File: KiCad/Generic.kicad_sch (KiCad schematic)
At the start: 39 parts, among them J1 Connector, J2 USB-C, J3 DC, U1 ESP32-WROOM-32, U2 FT231XQ, U3 LMR16006+FB

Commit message: Library tidy
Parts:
- D3, D4: footprint RevK:SOT-363_SC-70-6 -> Package_TO_SOT_SMD:SOT-363_SC-70-6
- U1: footprint RF_Module:ESP32-WROOM-32 -> RevK:ESP32-WROOM-32
- U2: footprint RevK:QFN-20-1EP_4x4mm_P0.5mm_EP2.5x2.5mm -> Package_DFN_QFN:QFN-20-1EP_4x4mm_P0.5mm_EP2.5x2.5mm
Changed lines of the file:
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@@
     (property "Reference" "U2" (id 0) (at 158.115 139.7 0))
     (property "Value" "FT231XQ" (id 1) (at 170.18 119.38 0))
-    (property "Footprint" "RevK:QFN-20-1EP_4x4mm_P0.5mm_EP2.5x2.5mm" (id 2) (at 205.105 138.43 0)
+    (property "Footprint" "Package_DFN_QFN:QFN-20-1EP_4x4mm_P0.5mm_EP2.5x2.5mm" (id 2) (at 205.105 138.43 0)
       (effects (font (size 1.27 1.27)) hide)
     )
@@
     (property "Reference" "D3" (id 0) (at 239.395 96.0882 0))
     (property "Value" "BAV99S" (id 1) (at 239.395 98.3996 0))
-    (property "Footprint" "RevK:SOT-363_SC-70-6" (id 2) (at 239.395 114.3 0)
+    (property "Footprint" "Package_TO_SOT_SMD:SOT-363_SC-70-6" (id 2) (at 239.395 114.3 0)
       (effects (font (size 1.27 1.27)) hide)
     )
@@
     (property "Reference" "D3" (id 0) (at 239.395 111.3282 0))
     (property "Value" "BAV99S" (id 1) (at 239.395 113.6396 0))
-    (property "Footprint" "RevK:SOT-363_SC-70-6" (id 2) (at 239.395 129.54 0)
+    (property "Footprint" "Package_TO_SOT_SMD:SOT-363_SC-70-6" (id 2) (at 239.395 129.54 0)
       (effects (font (size 1.27 1.27)) hide)
     )
@@
     (property "Reference" "D4" (id 0) (at 239.395 127.2032 0))
     (property "Value" "BAV99S" (id 1) (at 239.395 129.5146 0))
-    (property "Footprint" "RevK:SOT-363_SC-70-6" (id 2) (at 239.395 145.415 0)
+    (property "Footprint" "Package_TO_SOT_SMD:SOT-363_SC-70-6" (id 2) (at 239.395 145.415 0)
       (effects (font (size 1.27 1.27)) hide)
     )
@@
     (property "Reference" "D4" (id 0) (at 239.395 143.7132 0))
     (property "Value" "BAV99S" (id 1) (at 239.395 146.0246 0))
-    (property "Footprint" "RevK:SOT-363_SC-70-6" (id 2) (at 239.395 161.925 0)
+    (property "Footprint" "Package_TO_SOT_SMD:SOT-363_SC-70-6" (id 2) (at 239.395 161.925 0)
       (effects (font (size 1.27 1.27)) hide)
     )
@@
       (effects (font (size 1.27 1.27)) (justify left))
     )
-    (property "Footprint" "RF_Module:ESP32-WROOM-32" (id 2) (at 65.405 105.41 0)
+    (property "Footprint" "RevK:ESP32-WROOM-32" (id 2) (at 65.405 105.41 0)
       (effects (font (size 1.27 1.27)) hide)
     )
@@
     )
     (path "/00000000-0000-0000-0000-0000609f92b0"
-      (reference "D3") (unit 1) (value "BAV99S") (footprint "RevK:SOT-363_SC-70-6")
+      (reference "D3") (unit 1) (value "BAV99S") (footprint "Package_TO_SOT_SMD:SOT-363_SC-70-6")
     )
     (path "/00000000-0000-0000-0000-000060ddc5e7"
-      (reference "D3") (unit 2) (value "BAV99S") (footprint "RevK:SOT-363_SC-70-6")
+      (reference "D3") (unit 2) (value "BAV99S") (footprint "Package_TO_SOT_SMD:SOT-363_SC-70-6")
     )
     (path "/00000000-0000-0000-0000-000060ddef2c"
-      (reference "D4") (unit 1) (value "BAV99S") (footprint "RevK:SOT-363_SC-70-6")
+      (reference "D4") (unit 1) (value "BAV99S") (footprint "Package_TO_SOT_SMD:SOT-363_SC-70-6")
     )
     (path "/00000000-0000-0000-0000-000060de1009"
-      (reference "D4") (unit 2) (value "BAV99S") (footprint "RevK:SOT-363_SC-70-6")
+      (reference "D4") (unit 2) (value "BAV99S") (footprint "Package_TO_SOT_SMD:SOT-363_SC-70-6")
     )
     (path "/00000000-0000-0000-0000-0000610fe5d2"
@@
     )
     (path "/d3737146-f8f2-4cf9-a53d-a4805b531c09"
-      (reference "U1") (unit 1) (value "ESP32-WROOM-32") (footprint "RF_Module:ESP32-WROOM-32")
+      (reference "U1") (unit 1) (value "ESP32-WROOM-32") (footprint "RevK:ESP32-WROOM-32")
     )
     (path "/00000000-0000-0000-0000-000060849d1e"
-      (reference "U2") (unit 1) (value "FT231XQ") (footprint "RevK:QFN-20-1EP_4x4mm_P0.5mm_EP2.5x2.5mm")
+      (reference "U2") (unit 1) (value "FT231XQ") (footprint "Package_DFN_QFN:QFN-20-1EP_4x4mm_P0.5mm_EP2.5x2.5mm")
     )
     (path "/c88f1737-32b5-4cea-a76f-93ad322556d3"

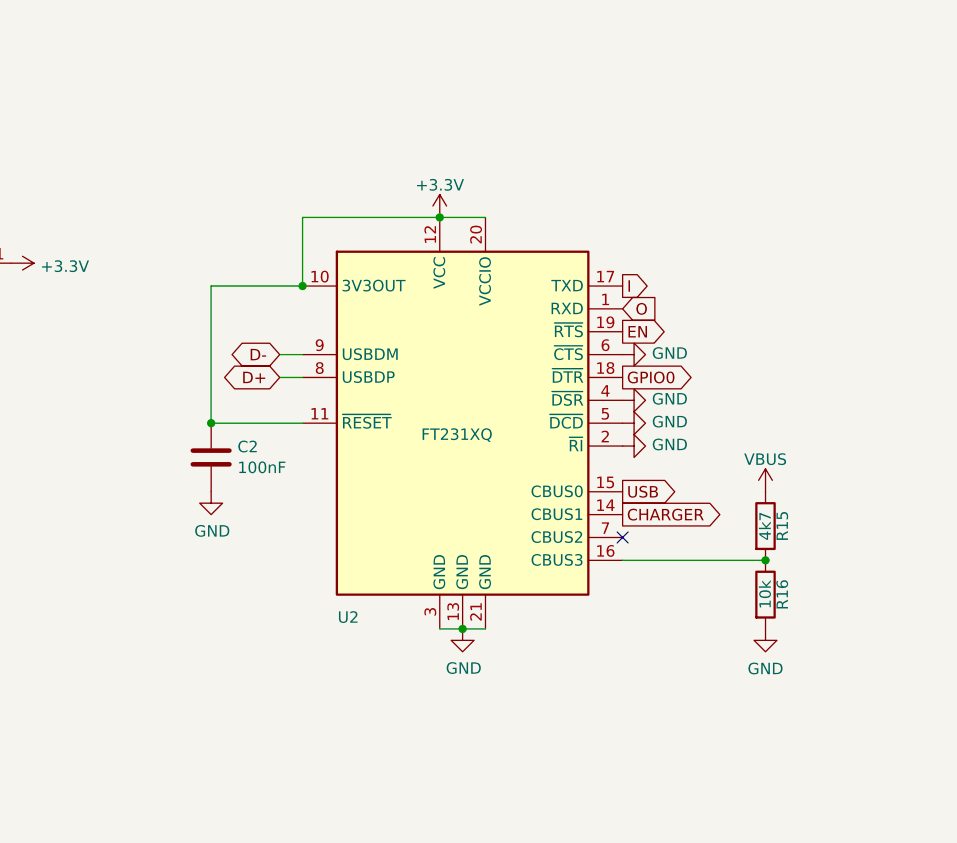
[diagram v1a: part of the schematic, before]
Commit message: Footprint update
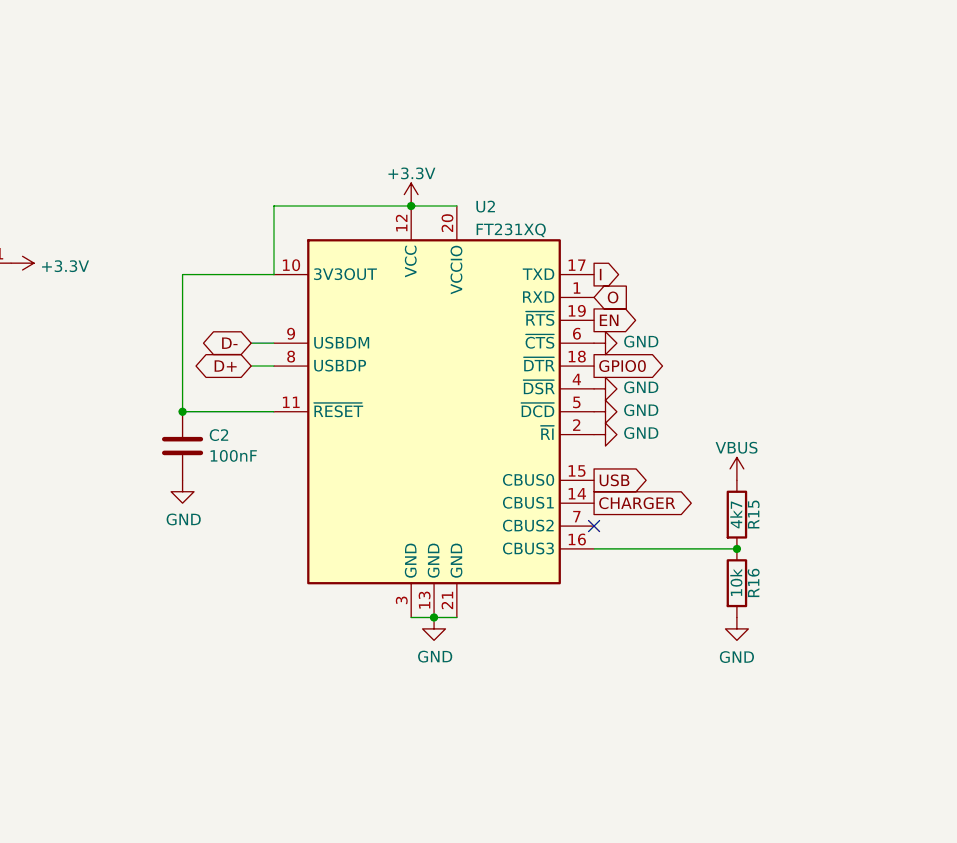
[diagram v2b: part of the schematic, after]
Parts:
- removed U2: FT231XQ, Package_DFN_QFN:QFN-20-1EP_4x4mm_P0.5mm_EP2.5x2.5mm, symbol Interface_USB:FT231XQ
- added U2: FT231XQ, RevK:QFN-20-1EP_4x4mm_P0.5mm_EP2.5x2.5mm, symbol RevK:FT231XQ
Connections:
- net +3V3: now also U2.10 (3V3OUT), U2.11 (~{RESET}), U2.12 (VCC), U2.20 (VCCIO)
- net CHARGER: now also U2.14 (CBUS1)
- net D+: now also U2.8 (USBDP)
- net D-: now also U2.9 (USBDM)
- net EN: now also U2.19 (~{RTS})
- net GND: now also U2.13 (GND), U2.2 (~{RI}), U2.21 (GND), U2.3 (GND), U2.4 (~{DSR}), U2.5 (~{DCD}), U2.6 (~{CTS})
- net GPIO0: now also U2.18 (~{DTR})
- net I: now also U2.17 (TXD)
- net O: now also U2.1 (RXD)
- net USB: now also U2.15 (CBUS0)
- net at R15.2, R16.1: now also U2.16 (CBUS3)
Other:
- moved on the sheet: C2, R15, R16
